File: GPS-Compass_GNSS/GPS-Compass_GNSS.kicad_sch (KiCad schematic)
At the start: 35 parts, among them J1 SMA_F, J3 01x10, Q1 MMBT3904, SW1 GNSS_RST, U1 BGA725L6E6327FTSA1, U2 TESEO-LIV3R

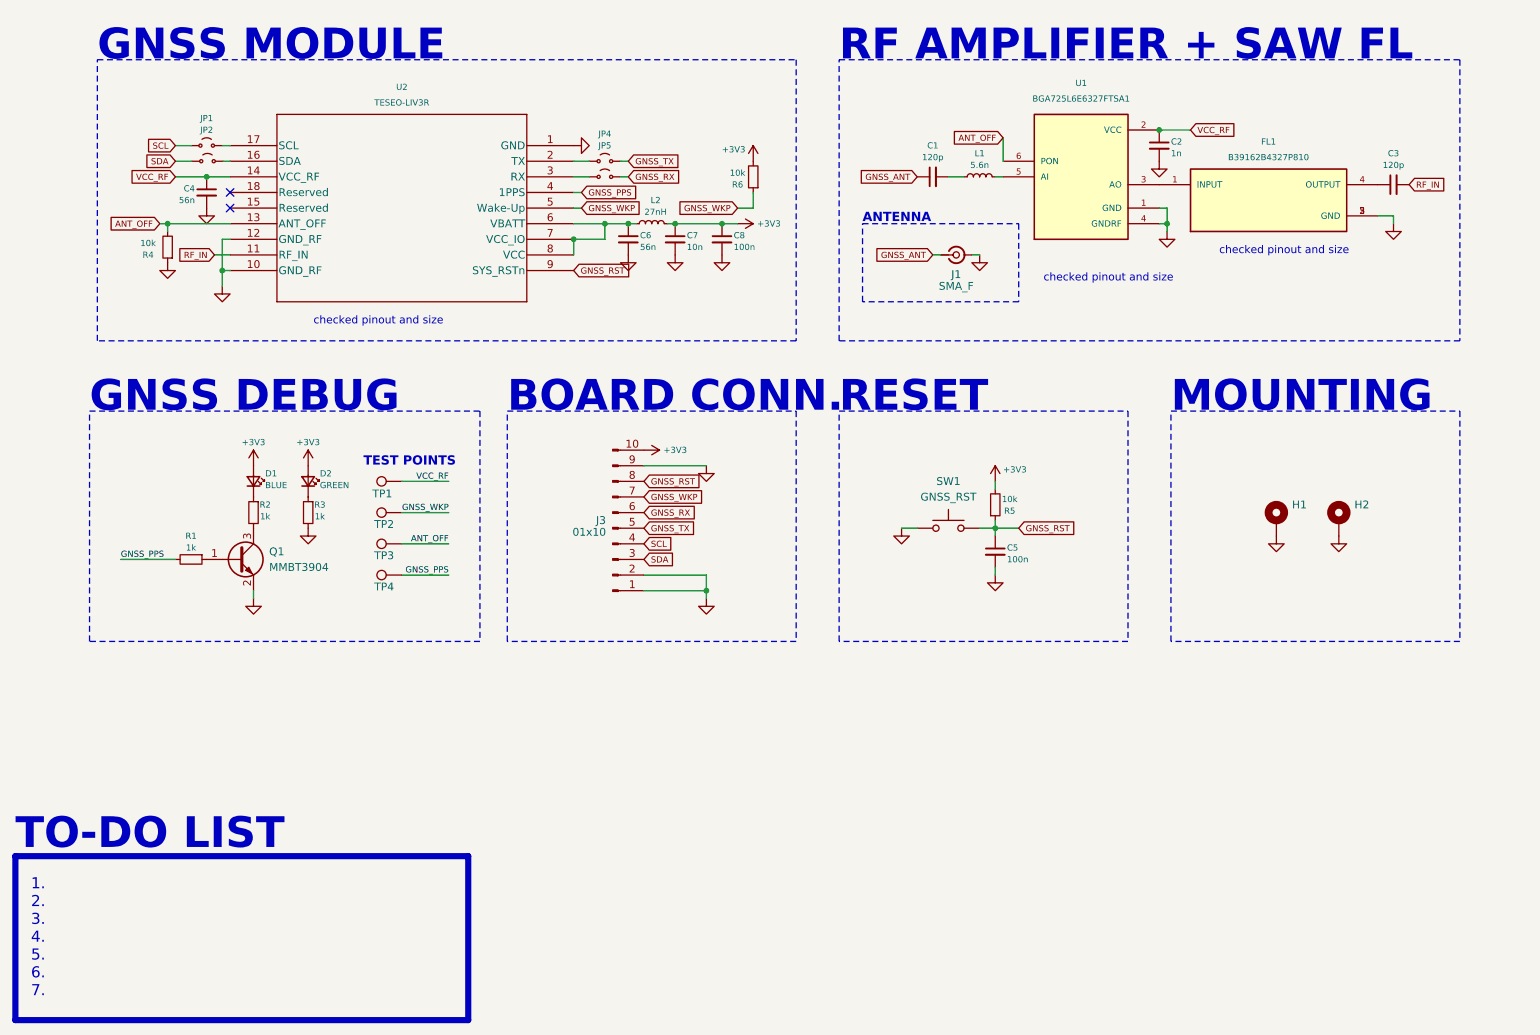
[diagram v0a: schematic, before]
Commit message: schematric remake
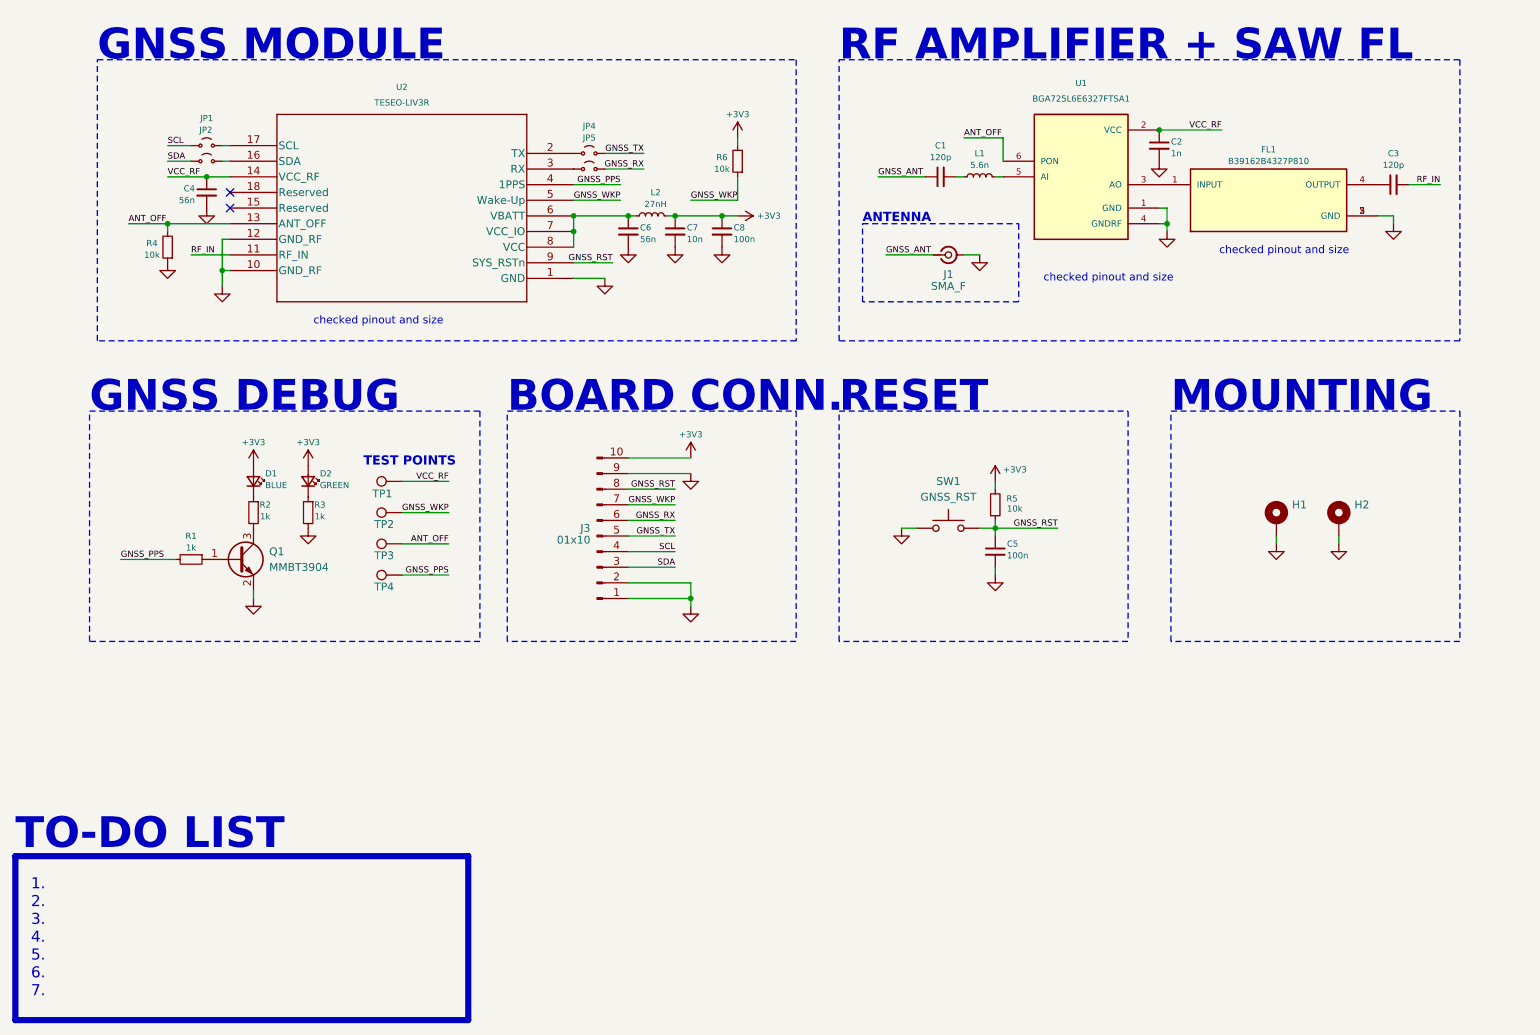
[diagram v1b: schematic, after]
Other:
- moved on the sheet: C1, C6, C7, C8, J1, J3, JP4, JP5, L2, R6
